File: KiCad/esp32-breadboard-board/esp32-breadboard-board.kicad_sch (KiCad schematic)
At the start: 24 parts, among them J2 Conn_01x22_Pin, J3 Conn_01x22_Pin, SW1 BOOT, SW2 EN, U1 ESP32-S3-WROOM-1, U2 USBLC6-2SC6, U3 SGM2212-3.3XKC3G

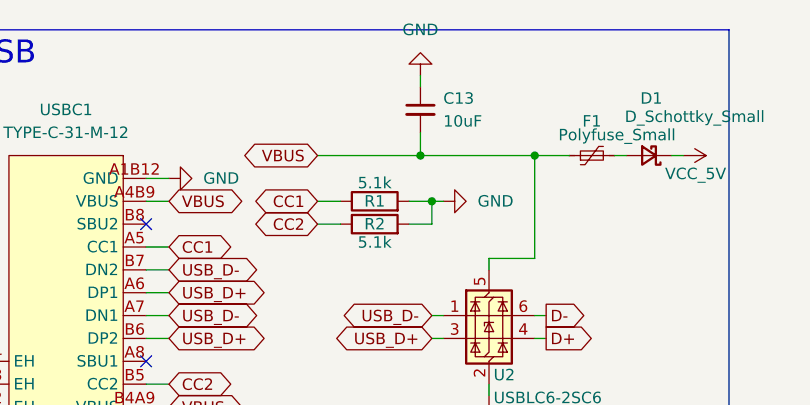
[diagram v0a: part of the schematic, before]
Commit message: commit
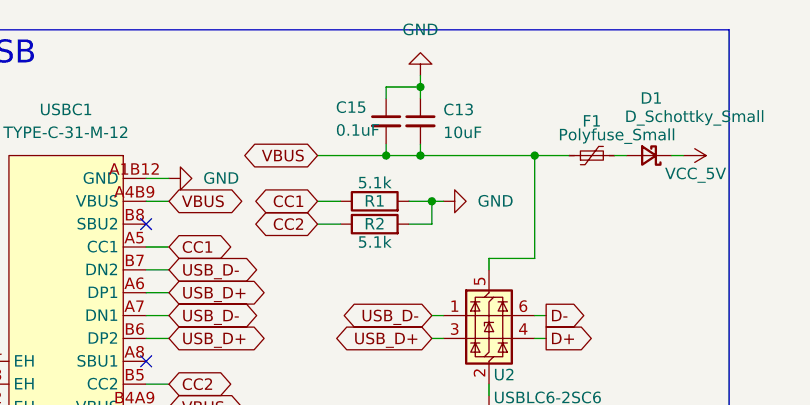
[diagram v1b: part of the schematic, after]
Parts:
- added C15: 0.1uF, Capacitor_SMD:C_0402_1005Metric, symbol Device:C_Small
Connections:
- net GND: now also C15.1
- net VBUS: now also C15.2
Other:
- moved on the sheet: C13
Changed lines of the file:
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@@
 	)
 	(junction
+		(at 68.58 31.75)
+		(diameter 0)
+		(color 0 0 0 0)
+	)
+	(junction
 		(at 120.65 96.52)
 		(diameter 0)
@@
 	)
 	(junction
+		(at 64.77 31.75)
+		(diameter 0)
+		(color 0 0 0 0)
+	)
+	(junction
 		(at 128.27 88.9)
 		(diameter 0)
@@
 	)
 	(junction
-		(at 81.28 31.75)
+		(at 68.58 24.13)
 		(diameter 0)
 		(color 0 0 0 0)
 	)
 	(junction
-		(at 68.58 31.75)
+		(at 81.28 31.75)
 		(diameter 0)
 		(color 0 0 0 0)
@@
 	(wire
 		(pts
+			(xy 64.77 31.75) (xy 68.58 31.75)
+		)
+		(stroke
+			(width 0)
+			(type default)
+		)
+	)
+	(wire
+		(pts
 			(xy 67.31 118.11) (xy 68.58 118.11)
 		)
@@
 	(wire
 		(pts
+			(xy 64.77 24.13) (xy 68.58 24.13)
+		)
+		(stroke
+			(width 0)
+			(type default)
+		)
+	)
+	(wire
+		(pts
 			(xy 251.46 96.52) (xy 255.27 96.52)
 		)
@@
 	(wire
 		(pts
-			(xy 68.58 29.21) (xy 68.58 31.75)
+			(xy 68.58 30.48) (xy 68.58 31.75)
 		)
 		(stroke
@@
 	(wire
 		(pts
+			(xy 64.77 25.4) (xy 64.77 24.13)
+		)
+		(stroke
+			(width 0)
+			(type default)
+		)
+	)
+	(wire
+		(pts
+			(xy 68.58 25.4) (xy 68.58 24.13)
+		)
+		(stroke
+			(width 0)
+			(type default)
+		)
+	)
+	(wire
+		(pts
 			(xy 120.65 88.9) (xy 128.27 88.9)
 		)
@@
 	(wire
 		(pts
+			(xy 64.77 30.48) (xy 64.77 31.75)
+		)
+		(stroke
+			(width 0)
+			(type default)
+		)
+	)
+	(wire
+		(pts
 			(xy 162.56 113.03) (xy 163.83 113.03)
 		)
@@
 	(wire
 		(pts
-			(xy 57.15 31.75) (xy 68.58 31.75)
+			(xy 57.15 31.75) (xy 64.77 31.75)
 		)
 		(stroke
@@
 	(symbol
 		(lib_id "Device:C_Small")
-		(at 68.58 26.67 0)
+		(at 68.58 27.94 0)
 		(unit 1)
 		(body_style 1)
@@
 		(fields_autoplaced yes)
 		(property "Reference" "C13"
-			(at 71.12 25.4062 0)
+			(at 71.12 26.6762 0)
 			(show_name no)
 			(do_not_autoplace no)
@@
 		)
 		(property "Value" "10uF"
-			(at 71.12 27.9462 0)
+			(at 71.12 29.2162 0)
 			(show_name no)
 			(do_not_autoplace no)
@@
 		)
 		(property "Footprint" "Capacitor_SMD:C_0603_1608Metric"
-			(at 68.58 26.67 0)
+			(at 68.58 27.94 0)
 			(hide yes)
 			(show_name no)
@@
 		)
 		(property "Datasheet" ""
-			(at 68.58 26.67 0)
+			(at 68.58 27.94 0)
 			(hide yes)
 			(show_name no)
@@
 		)
 		(property "Description" "Unpolarized capacitor, small symbol"
-			(at 68.58 26.67 0)
+			(at 68.58 27.94 0)
 			(hide yes)
 			(show_name no)
@@
 					(unit 1)
 				)
+			)
+		)
+	)
+	(symbol
+		(lib_id "Device:C_Small")
+		(at 64.77 27.94 0)
+		(unit 1)
+		(body_style 1)
+		(exclude_from_sim no)
+		(in_bom yes)
+		(on_board yes)
+		(in_pos_files yes)
+		(dnp no)
+		(property "Reference" "C15"
+			(at 59.182 26.416 0)
+			(show_name no)
+			(do_not_autoplace no)
+			(effects
+				(font
+					(size 1.27 1.27)
+				)
+				(justify left)
+			)
+		)
+		(property "Value" "0.1uF"
+			(at 59.182 28.956 0)
+			(show_name no)
+			(do_not_autoplace no)
+			(effects
+				(font
+					(size 1.27 1.27)
+				)
+				(justify left)
+			)
+		)
+		(property "Footprint" "Capacitor_SMD:C_0402_1005Metric"
+			(at 64.77 27.94 0)
+			(hide yes)
+			(show_name no)
+			(do_not_autoplace no)
+			(effects
+				(font
+					(size 1.27 1.27)
+				)
+			)
+		)
+		(property "Datasheet" ""
+			(at 64.77 27.94 0)
+			(hide yes)
+			(show_name no)
+			(do_not_autoplace no)
+			(effects
+				(font
+					(size 1.27 1.27)
+				)
+			)
+		)
+		(property "Description" "Unpolarized capacitor, small symbol"
+			(at 64.77 27.94 0)
+			(hide yes)
+			(show_name no)
+			(do_not_autoplace no)
+			(effects
+				(font
+					(size 1.27 1.27)
+				)
+			)
+		)
+		(pin "2"
+		)
+		(pin "1"
+		)
+		(instances
+			(project "esp32-breadboard-board"
+				(path "/e775903e-c2eb-40b7-aba5-14dc5f95329e"
+					(reference "C15")
+					(unit 1)
+				)

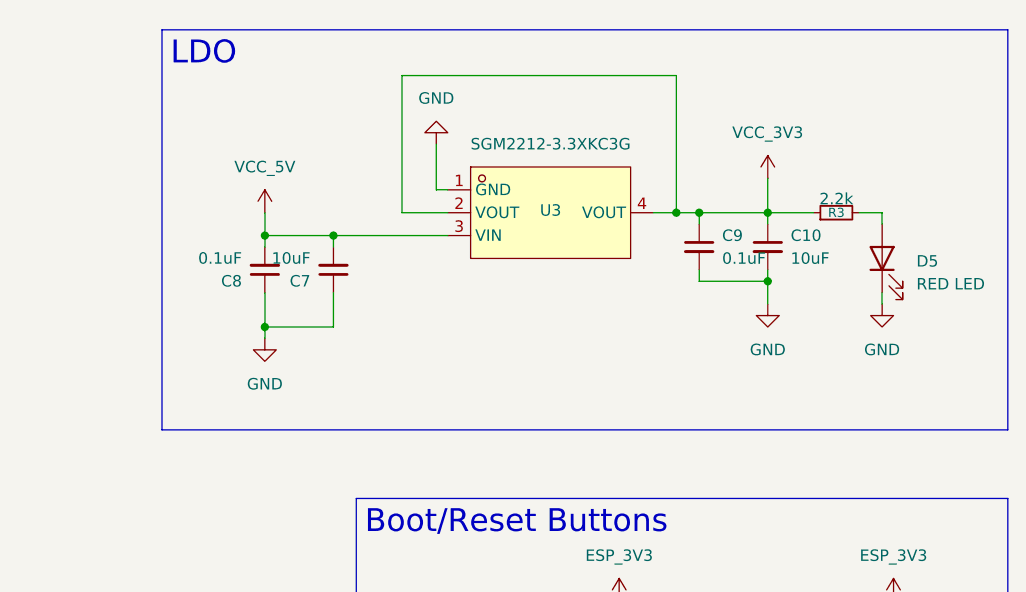
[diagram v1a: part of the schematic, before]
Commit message: Updated BOM
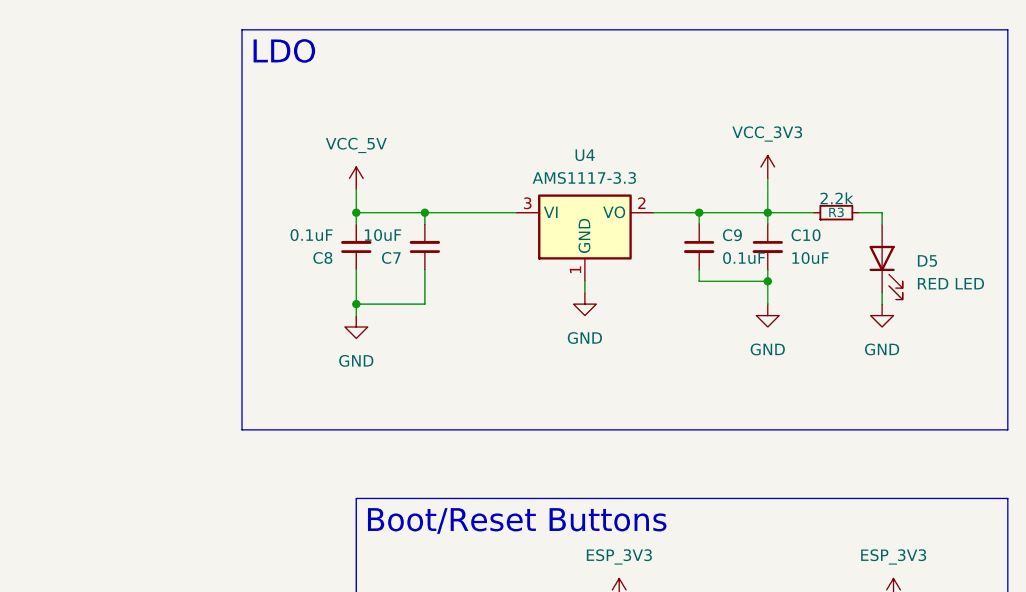
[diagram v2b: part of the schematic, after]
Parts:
- removed U3: SGM2212-3.3XKC3G, easyeda2kicad:SOT-223-3_L6.5-W3.4-P2.30-LS7.0-BR, symbol easyeda2kicad:SGM2212-3.3XKC3G_TR_C3294699
- added U4: AMS1117-3.3, Package_TO_SOT_SMD:SOT-223-3_TabPin2, symbol Regulator_Linear:AMS1117-3.3
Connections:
- net ESP_3V3: now also U4.2 (VO)
- net GND: now also U4.1 (GND)
- net VCC_5V: now also U4.3 (VI)
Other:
- moved on the sheet: C7, C8
